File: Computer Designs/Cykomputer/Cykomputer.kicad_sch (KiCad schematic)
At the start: 77 parts, among them J1 Bus_ISA_8bit, J10 DE15_Socket_HighDensity_Mount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, J11 USB_C_Receptacle, J12 IEC_60320_C14_Receptacle, J13 Conn_01x02, J14 PINHD_1x2_Male, J15 Bus_ISA_8bit, J16 Conn_02x12_Row_Letter_First, J17 Conn_01x12, J18 AudioJack2, J19 Conn_01x32, J2 Bus_ISA_8bit, J20 Conn_01x09, J3 Bus_ISA_8bit, J4 DE9_Pins_MountingHoles, J5 DE9_Pins_MountingHoles, J6 Mini-DIN-6, J7 DE15_Socket_HighDensity_Mount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, J8 DE15_Socket_HighDensity_Mount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, J9 DE15_Socket_HighDensity_Mount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, SW1 SW_SPST, SW2 SW_Rotary_1x7_MP, SW3 Push_Button, U1 W65C02SxP, U10 74HC14, U11 W65C51NxP, U12 W65C02SxP, U13 27C256, U14 KM62256CLP, U15 KM62256CLP, U16 27C256, U17 74HCT595, U18 74HCT164, U19 KM62256CLP, U2 74LS30, U20 4053, U21 MIC2025-2YM, U22 W65C22SxP, U23 74HCT595, U24 74HCT595, U25 KM62256CLP, U26 W65C22SxP, U27 CH340G, U28 DS1813-5, U29 CH376S, U30 6581, U4 W65C22SxP, U5 W65C51NxP, U6 W65C51NxP, U7 MAX232, U8 MAX232, U9 W65C22SxP, Y1 ACO-xxxMHz-A, Y2 ACO-xxxMHz-A, Y3 ACO-xxxMHz-A, Y4 ACO-xxxMHz-A, Y5 ACO-xxxMHz-A, Y6 ACO-xxxMHz-A, Y7 ACO-xxxMHz-A

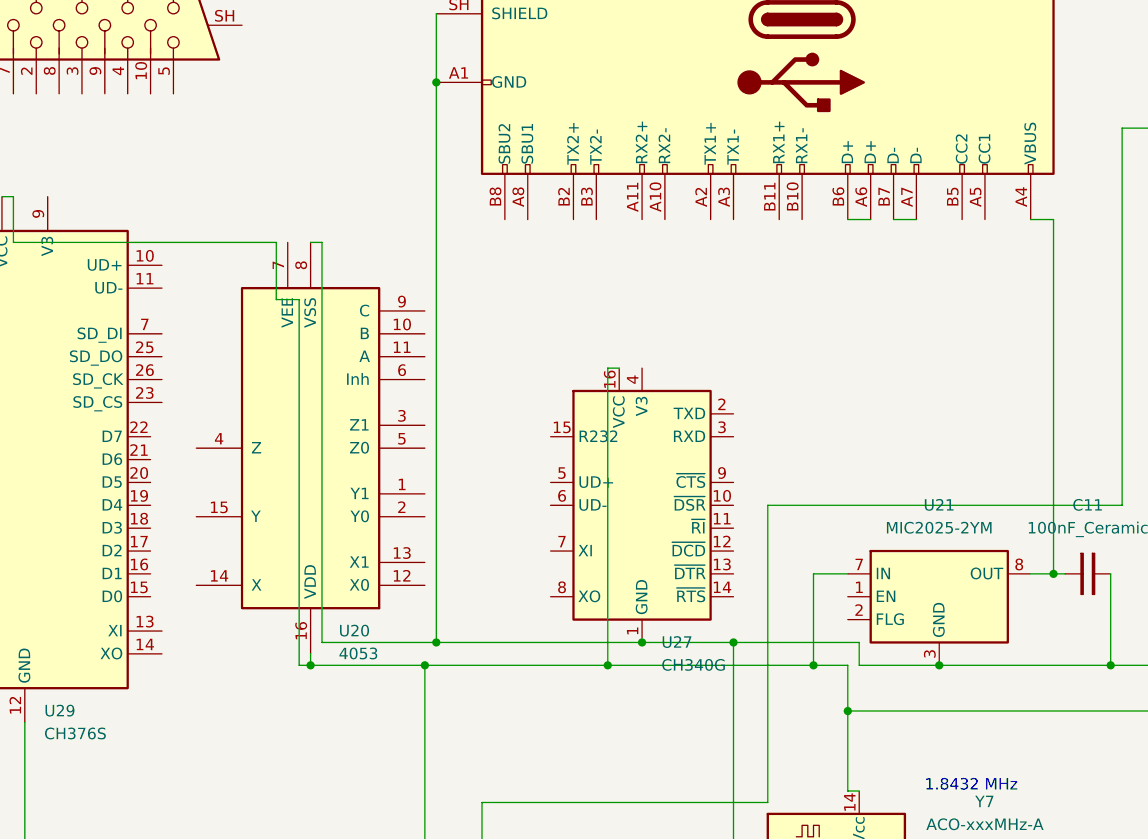
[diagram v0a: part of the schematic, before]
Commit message: Finished Keyboard Design
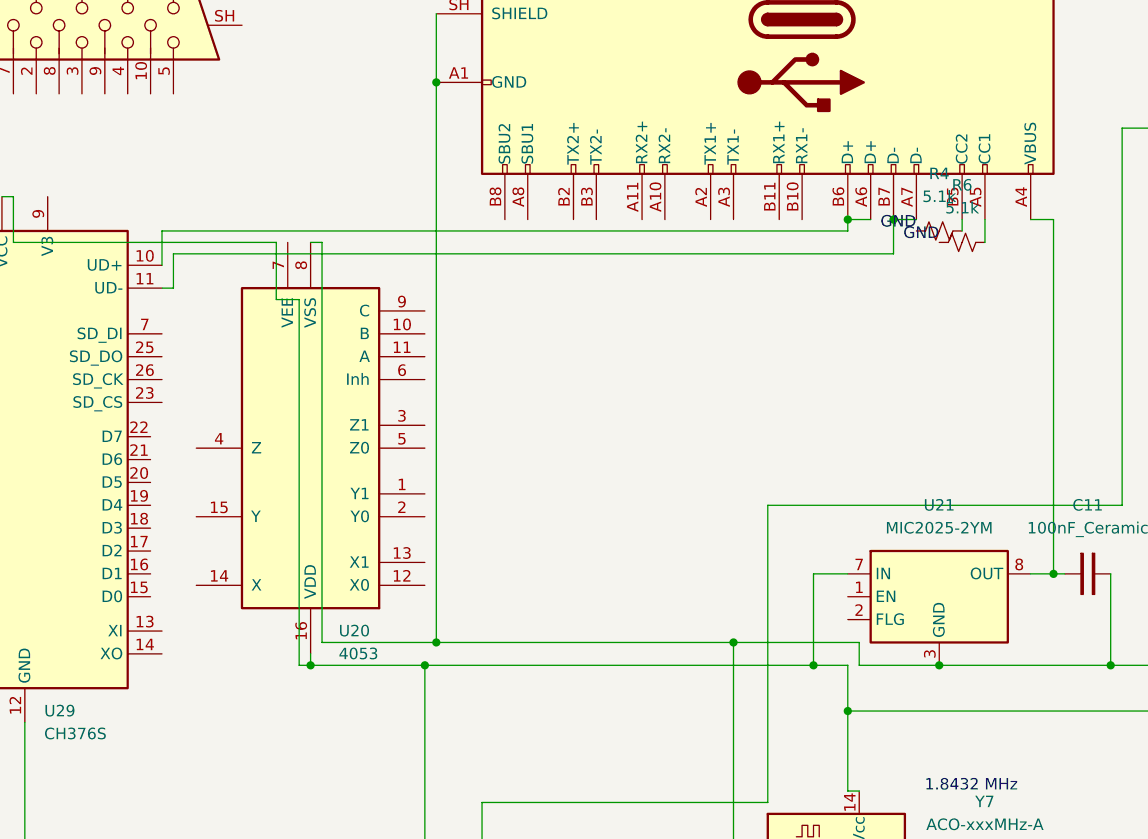
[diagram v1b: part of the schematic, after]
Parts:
- removed U27: CH340G, Package_SO:SOIC-16_3.9x9.9mm_P1.27mm, symbol Interface_USB:CH340G
- added R4, R6: 5.1k, PCM_4ms_Resistor:R_Axial_DIN0207_L6.3mm_D2.5mm_P7.62mm_Horizontal, symbol PCM_SparkFun-Resistor:5.1k_0603
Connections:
- net GND: now also R4.1, R6.1
- net at J11.A5 (CC1): now also R6.2
- net at J11.A6 (D+), J11.B6 (D+): now also U29.10 (UD+)
- net at J11.A7 (D-), J11.B7 (D-): now also U29.11 (UD-)
- net at J11.B5 (CC2): now also R4.2
